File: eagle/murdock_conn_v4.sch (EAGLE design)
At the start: 12 parts, among them X7 MURDOCK_STACK

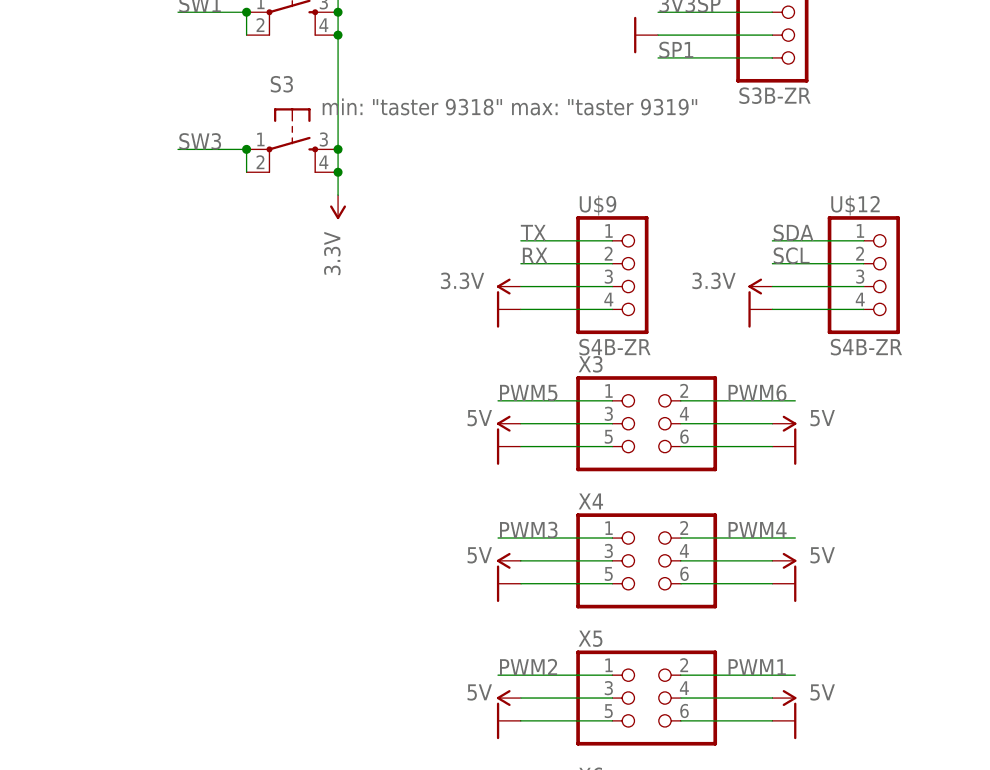
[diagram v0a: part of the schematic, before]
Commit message: v4
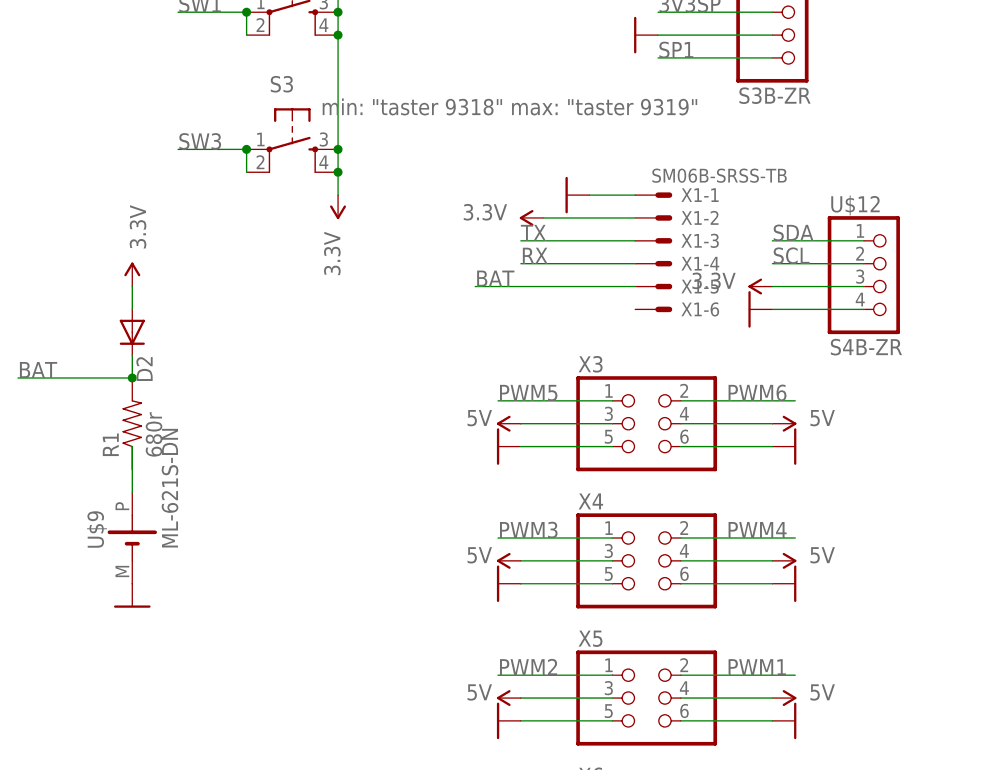
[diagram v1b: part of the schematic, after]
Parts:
- added D2: (no value), diode:DIODE-SOD323-R
- added R1: 680r, SparkFun-Passives:RESISTOR0805-RES
- added X1: SM06B-SRSS-TB, con-jst:SM06B-SRSS-TB
- U$9: value S4B-ZR -> ML-621S-DN; device seb:S4B-ZR -> seb:ML-621S-DN
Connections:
- new net BAT: D2.C, R1.2, X1-5.S
- new net N$1: R1.1, U$9.+
- net 3.3V: now also D2.A, X1-2.S; no longer U$9.3
- net GND: now also U$9.-, X1-1.S; no longer U$9.4
- net RX: now also X1-4.S; no longer U$9.2
- net TX: now also X1-3.S; no longer U$9.1
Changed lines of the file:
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@@
 <part name="X7" library="murdock" deviceset="MURDOCK_STACK" device=""/>
 <part name="P+3" library="SparkFun-Aesthetics" deviceset="3.3V" device=""/>
-<part name="U$9" library="seb" deviceset="S4B-ZR" device=""/>
 <part name="U$12" library="seb" deviceset="S4B-ZR" device=""/>
+<part name="X1" library="con-jst" deviceset="?M06B-SRSS-TB" device="S"/>
+<part name="R1" library="SparkFun-Passives" deviceset="RESISTOR" device="0805-RES" value="680r"/>
+<part name="P+4" library="SparkFun-Aesthetics" deviceset="3.3V" device=""/>
+<part name="GND11" library="supply1" deviceset="GND" device=""/>
+<part name="U$9" library="seb" deviceset="ML-621S-DN" device=""/>
+<part name="D2" library="diode" deviceset="DIODE-" device="SOD323-R"/>
 </parts>
 <sheets>
@@
 <attribute name="VALUE" x="9.144" y="45.466" size="1.778" layer="96"/>
 </instance>
-<instance part="P+1" gate="G$1" x="15.24" y="76.2" smashed="yes" rot="R90">
-<attribute name="VALUE" x="11.176" y="77.724" size="1.778" layer="96" rot="R180"/>
-</instance>
-<instance part="GND9" gate="1" x="12.7" y="73.66" smashed="yes" rot="R270"/>
+<instance part="P+1" gate="G$1" x="17.78" y="83.82" smashed="yes" rot="R90">
+<attribute name="VALUE" x="13.716" y="85.344" size="1.778" layer="96" rot="R180"/>
+</instance>
+<instance part="GND9" gate="1" x="20.32" y="86.36" smashed="yes" rot="R270"/>
 <instance part="P+2" gate="G$1" x="43.18" y="76.2" smashed="yes" rot="R90">
 <attribute name="VALUE" x="39.116" y="77.724" size="1.778" layer="96" rot="R180"/>
@@
 <attribute name="VALUE" x="-6.604" y="82.296" size="1.778" layer="96" rot="R270"/>
 </instance>
-<instance part="U$9" gate="G$1" x="25.4" y="76.2"/>
 <instance part="U$12" gate="G$1" x="53.34" y="76.2"/>
+<instance part="X1" gate="-1" x="30.48" y="86.36"/>
+<instance part="X1" gate="-2" x="30.48" y="83.82"/>
+<instance part="X1" gate="-3" x="30.48" y="81.28"/>
+<instance part="X1" gate="-4" x="30.48" y="78.74"/>
+<instance part="X1" gate="-5" x="30.48" y="76.2"/>
+<instance part="X1" gate="-6" x="30.48" y="73.66"/>
+<instance part="R1" gate="G$1" x="-27.94" y="60.96" rot="R90"/>
+<instance part="P+4" gate="G$1" x="-27.94" y="76.2" smashed="yes">
+<attribute name="VALUE" x="-26.416" y="80.264" size="1.778" layer="96" rot="R90"/>
+</instance>
+<instance part="GND11" gate="1" x="-27.94" y="40.64" smashed="yes"/>
+<instance part="U$9" gate="G$1" x="-27.94" y="48.26" rot="R90"/>
+<instance part="D2" gate="G$1" x="-27.94" y="71.12" rot="R270"/>
 </instances>
 <busses>
@@
 <segment>
 <pinref part="GND9" gate="1" pin="GND"/>
-<wire x1="15.24" y1="73.66" x2="25.4" y2="73.66" width="0.1524" layer="91"/>
-<pinref part="U$9" gate="G$1" pin="4"/>
+<wire x1="22.86" y1="86.36" x2="27.94" y2="86.36" width="0.1524" layer="91"/>
+<pinref part="X1" gate="-1" pin="S"/>
 </segment>
 <segment>
@@
 <label x="116.84" y="88.9" size="1.778" layer="95"/>
 </segment>
+<segment>
+<pinref part="GND11" gate="1" pin="GND"/>
+<pinref part="U$9" gate="G$1" pin="-"/>
+</segment>
 </net>
 <net name="5V" class="0">
@@
 <segment>
 <pinref part="P+1" gate="G$1" pin="3.3V"/>
-<wire x1="15.24" y1="76.2" x2="25.4" y2="76.2" width="0.1524" layer="91"/>
-<pinref part="U$9" gate="G$1" pin="3"/>
+<wire x1="17.78" y1="83.82" x2="27.94" y2="83.82" width="0.1524" layer="91"/>
+<pinref part="X1" gate="-2" pin="S"/>
 </segment>
 <segment>
@@
 <pinref part="P+3" gate="G$1" pin="3.3V"/>
 </segment>
+<segment>
+<pinref part="P+4" gate="G$1" pin="3.3V"/>
+<wire x1="-27.94" y1="76.2" x2="-27.94" y2="73.66" width="0.1524" layer="91"/>
+<pinref part="D2" gate="G$1" pin="A"/>
+</segment>
 </net>
 <net name="SDA" class="0">
@@
 </segment>
 <segment>
-<wire x1="25.4" y1="78.74" x2="15.24" y2="78.74" width="0.1524" layer="91"/>
+<wire x1="27.94" y1="78.74" x2="15.24" y2="78.74" width="0.1524" layer="91"/>
 <label x="15.24" y="78.74" size="1.778" layer="95"/>
-<pinref part="U$9" gate="G$1" pin="2"/>
+<pinref part="X1" gate="-4" pin="S"/>
 </segment>
 </net>
@@
 </segment>
 <segment>
-<wire x1="25.4" y1="81.28" x2="15.24" y2="81.28" width="0.1524" layer="91"/>
+<wire x1="27.94" y1="81.28" x2="15.24" y2="81.28" width="0.1524" layer="91"/>
 <label x="15.24" y="81.28" size="1.778" layer="95"/>
-<pinref part="U$9" gate="G$1" pin="1"/>
+<pinref part="X1" gate="-3" pin="S"/>
 </segment>
 </net>
@@
 </segment>
 </net>
+<net name="BAT" class="0">
+<segment>
+<pinref part="X1" gate="-5" pin="S"/>
+<wire x1="27.94" y1="76.2" x2="10.16" y2="76.2" width="0.1524" layer="91"/>
+<label x="10.16" y="76.2" size="1.778" layer="95"/>
+</segment>
+<segment>
+<pinref part="R1" gate="G$1" pin="2"/>
+<wire x1="-27.94" y1="66.04" x2="-40.64" y2="66.04" width="0.1524" layer="91"/>
+<junction x="-27.94" y="66.04"/>
+<label x="-40.64" y="66.04" size="1.778" layer="95"/>
+<pinref part="D2" gate="G$1" pin="C"/>
+<wire x1="-27.94" y1="66.04" x2="-27.94" y2="68.58" width="0.1524" layer="91"/>
+</segment>
+</net>
+<net name="N$1" class="0">
+<segment>
+<pinref part="R1" gate="G$1" pin="1"/>
+<wire x1="-27.94" y1="55.88" x2="-27.94" y2="58.42" width="0.1524" layer="91"/>
+<wire x1="-27.94" y1="55.88" x2="-27.94" y2="53.34" width="0.1524" layer="91"/>
+<pinref part="U$9" gate="G$1" pin="+"/>
+</segment>
+</net>
